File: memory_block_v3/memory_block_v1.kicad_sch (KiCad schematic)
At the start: 19 parts, among them J1 4677, J11 Conn_01x07, J2 DM3D-SF, J3 Conn_01x02, J4 Conn_01x19, J5 Conn_01x03, J6 Conn_01x19, J7 Conn_02x04_Top_Bottom, U1 ESP32-WROOM-32E-N8, U2 W25Q128JVSIQ TR

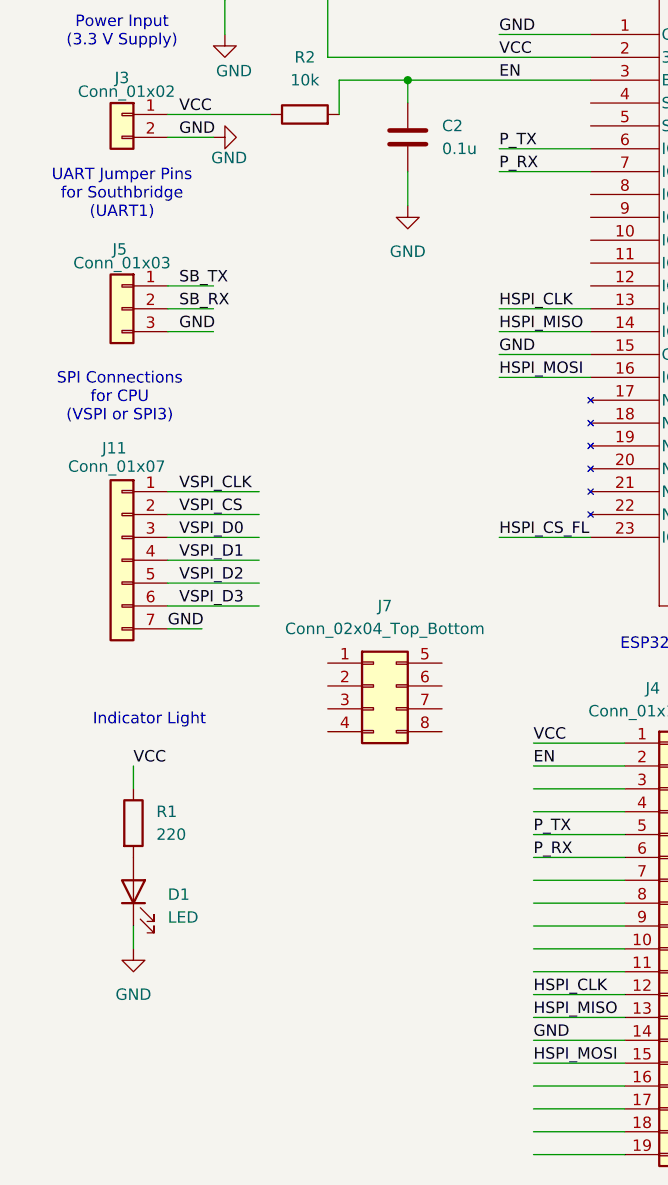
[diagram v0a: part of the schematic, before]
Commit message: continued NB/MB pcb progress
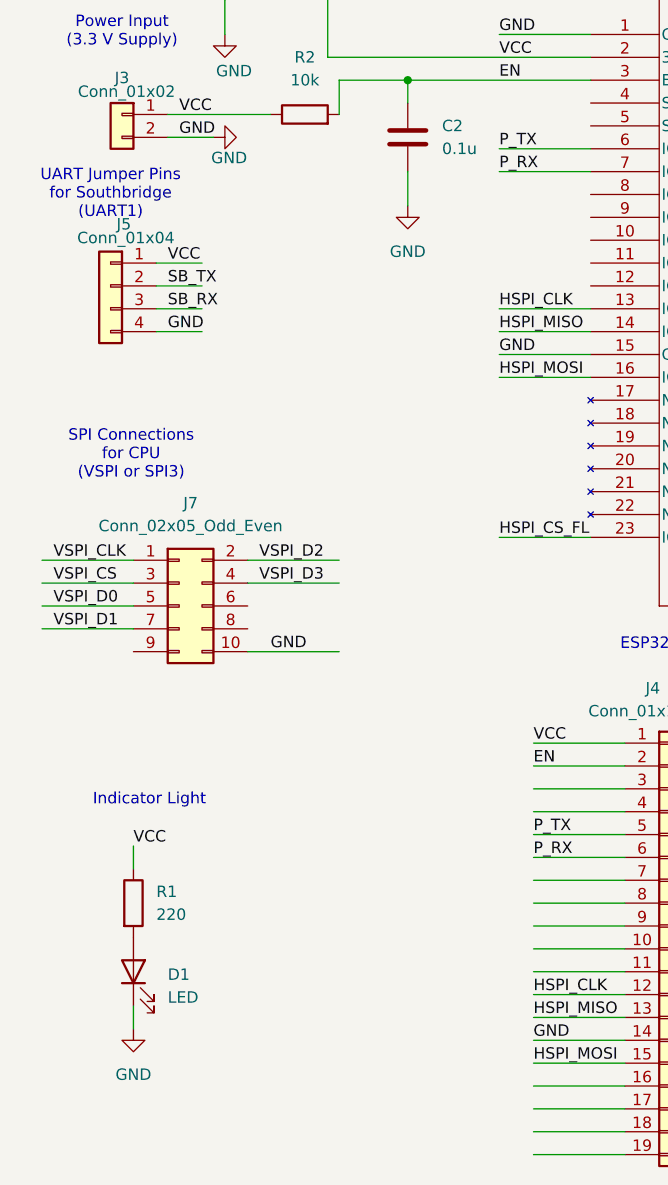
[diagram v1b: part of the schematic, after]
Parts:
- removed J11: Conn_01x07, Connector_PinSocket_2.54mm:PinSocket_1x07_P2.54mm_Horizontal, symbol Connector_Generic:Conn_01x07
- removed J5: Conn_01x03, Connector_PinSocket_2.54mm:PinSocket_1x03_P2.54mm_Vertical, symbol Connector_Generic:Conn_01x03
- removed J7: Conn_02x04_Top_Bottom, symbol Connector_Generic:Conn_02x04_Top_Bottom
- added J5: Conn_01x04, Connector_PinHeader_2.54mm:PinHeader_1x04_P2.54mm_Horizontal, symbol Connector_Generic:Conn_01x04
- added J7: Conn_02x05_Odd_Even, Connector_PinHeader_2.54mm:PinHeader_2x05_P2.54mm_Horizontal, symbol Connector_Generic:Conn_02x05_Odd_Even
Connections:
- net GND: now also J5.1 (Pin_1), J5.2 (Pin_2), J5.3 (Pin_3), J5.4 (Pin_4), J7.1 (Pin_1), J7.10 (Pin_10), J7.2 (Pin_2), J7.3 (Pin_3), J7.4 (Pin_4), J7.5 (Pin_5), J7.7 (Pin_7)
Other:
- moved on the sheet: D1, R1
